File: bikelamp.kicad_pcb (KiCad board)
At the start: 2 copper layers, 56.5 x 60.1 mm, 71 parts, among them J1 Conn_ARM_SWD_TagConnect_TC203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, Q1 Q_PMOS_GSD, Q2 BSS138, Q3 RBFET, Q4 HIGH, Q5 LOW, Q6 ACFET, Q7 BSS138, Q8 YJQ3400A-YAN, Q9 YJQ3400A-YAN, SW1 SW_MEC_5E, U1 MCP79402T-xSN, U2 BQ24780SRUYR, U3 MIC5205-3.3YM5, U4 MMA8452QR1, U5 YJ-14015, U6 MC-306

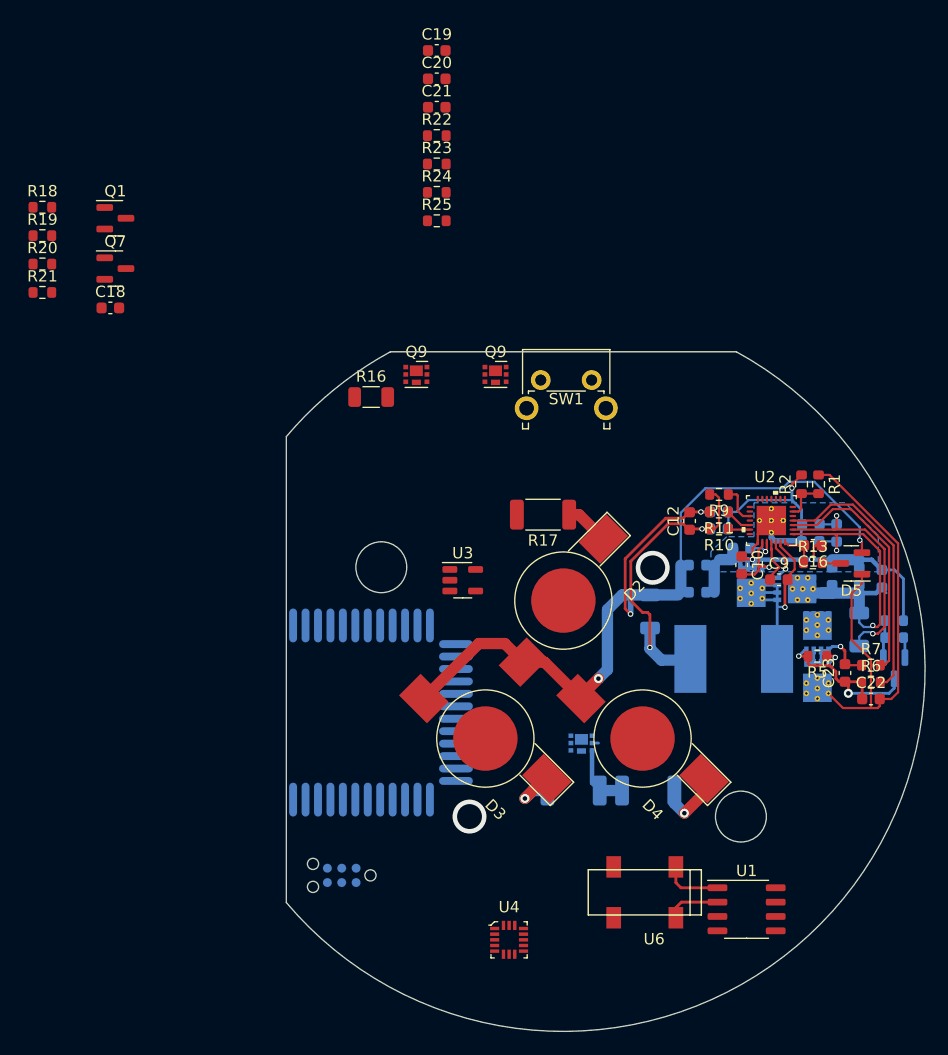
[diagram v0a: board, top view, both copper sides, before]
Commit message: Board routed
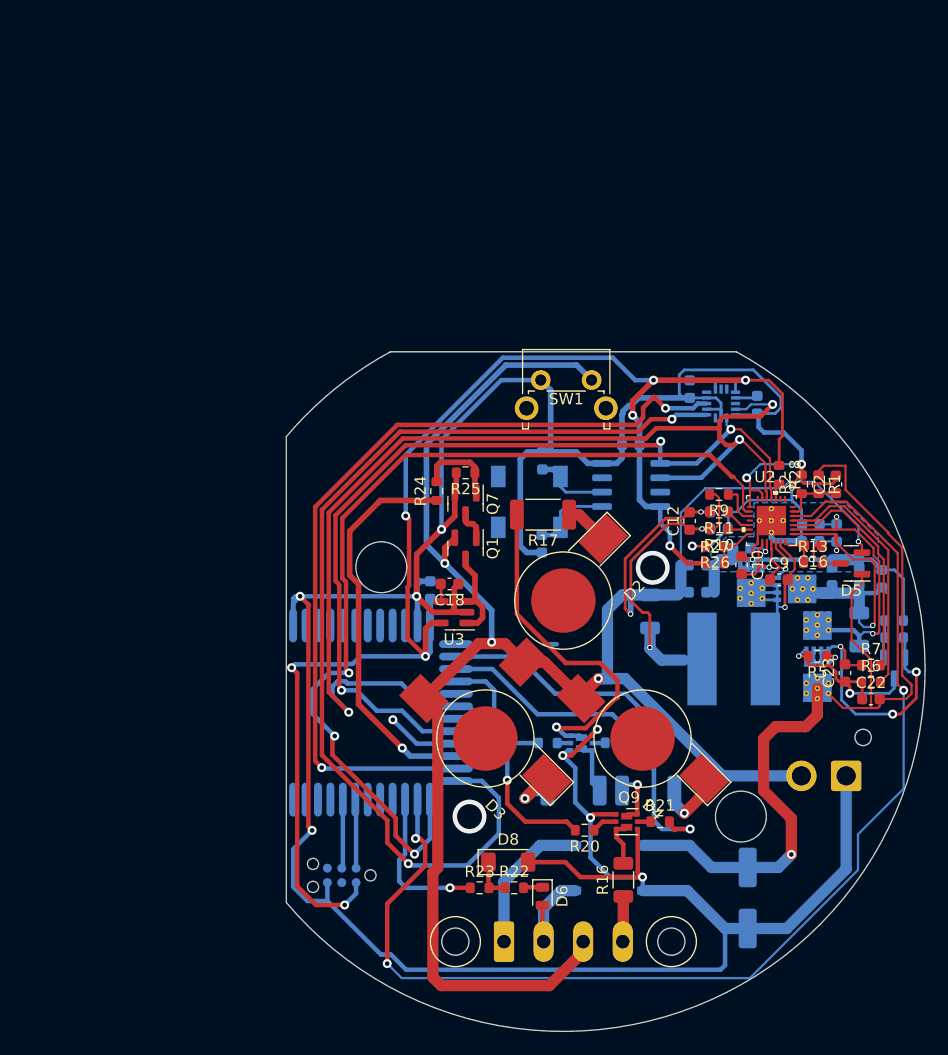
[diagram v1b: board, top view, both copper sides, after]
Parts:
- removed the Q9 at (-3.00, 2.00)
- removed the Q9 at (4.00, 2.00)
- added C1: 100uF, Capacitor_SMD:CP_Elec_6.3x5.7, B.Cu at (26.3, 48.3)
- added C2: 100nF, Capacitor_SMD:C_0603_1608Metric, F.Cu at (34.1, 11.7)
- added C24: 100nF, Capacitor_SMD:C_0603_1608Metric, B.Cu at (21.2, 3.30)
- added C25: 100nF, Capacitor_SMD:C_0603_1608Metric, B.Cu at (16.0, 8.23)
- added C26: 100nF, Capacitor_SMD:C_0603_1608Metric, B.Cu at (-1.77, 21.1)
- added D1: D_Bridge_+-AA, Diode_SMD:Diode_Bridge_Diotec_ABS, B.Cu at (14.1, 45.6)
- added D6: D_Schottky, Diode_SMD:D_MicroMELF, F.Cu at (8.15, 48.1)
- added D8: BZV55C2V7, Diode_SMD:D_MiniMELF, F.Cu at (5.12, 45.1)
- added J2: Conn_01x04_Pin, Connector_Phoenix_MC:PhoenixContact_MCV_1,5_4-GF-3.5_1x04_P3.50mm_Vertical_ThreadedFlange_MountHole, B.Cu at (4.75, 52.2)
- added J_BATTERY1: Conn_01x02, Connector_JST:JST_VH_B2P-VH-FB-B_1x02_P3.96mm_Vertical, B.Cu at (35.0, 37.5)
- added Q9: YJQ3400A-YAN, footprints:DFN2020-6L, F.Cu at (15.6, 41.5)
- added R26: TBD, Resistor_SMD:R_0603_1608Metric, F.Cu at (23.4, 17.2)
- added R27: TBD, Resistor_SMD:R_0603_1608Metric, F.Cu at (23.4, 18.7)
- added R28: 10K, Resistor_SMD:R_0603_1608Metric, F.Cu at (29.1, 10.9)
- C19, C20, C21, R18, R19, U1, U6: moved to B.Cu
- L1: footprint libs:IND_ETQP5M150YFK -> Inductor_SMD:L_Bourns-SRN8040_8x8.15mm
- Q8: footprint Package_DFN_QFN:Diodes_UDFN2020-6_Type-F -> footprints:DFN2020-6L
- U4: footprint digikey-footprints:VQFN-16_3x3mm -> footprints:VQFN-16_3x3mm; moved to B.Cu
- moved R21 71.9 mm to (18.6, 41.5)
- moved R20 69.3 mm to (11.9, 42.3), turned to 180 degrees
- moved R18 69.3 mm to (14.5, 34.6)
- moved R22 66.9 mm to (5.65, 47.4)
- moved R23 64.1 mm to (2.60, 47.4)
- moved R19 63.3 mm to (8.62, 34.6), turned to 180 degrees
- moved U4 51.0 mm to (23.9, 4.58), turned to 180 degrees
- moved R16 48.2 mm to (15.3, 46.7), turned to 90 degrees
- moved Q1 42.6 mm to (1.35, 17.4), turned to -90 degrees
- moved C19 42.2 mm to (27.1, 4.67), turned to 90 degrees
- moved C21 39.7 mm to (8.09, 17.0), turned to 90 degrees
- moved U1 38.9 mm to (16.0, 11.8)
- moved C18 38.7 mm to (-0.07, 20.5), turned to 180 degrees
- moved Q7 37.3 mm to (1.35, 13.4), turned to -90 degrees
- moved U6 36.0 mm to (6.99, 13.3)
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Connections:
- net /BQ24780/ACN renamed /BQ24780/VIN_I_MEASURED
- net /BQ24780/ACP renamed /BQ24780/VIN_REVPROT
- R16 pad 1: Net-(J_REAR_LAMP1-Pin_1) -> REAR_LAMP_K
- U2 pad 10: unconnected-(U2-PROCHOT_N-Pad10) -> Net-(U2-PROCHOT_N)
- U2 pad 13: unconnected-(U2-CMPIN-Pad13) -> GND
- U2 pad 15: unconnected-(U2-BATPRES_N-Pad15) -> GND
- U2 pad 16: unconnected-(U2-TB_STAT_N-Pad16) -> TB_STAT
- U2 pad 21: unconnected-(U2-ILIM-Pad21) -> /BQ24780/ILIM
- U2 pad 5: unconnected-(U2-ACOK-Pad5) -> ACOK
- U5 pad 15: LED_PWM_1 -> LED_PWM_0
- U5 pad 16: LED_PWM_0 -> LED_PWM_1
- U5 pad 17: WHEEL_SIGNAL -> unconnected-(U5-P03-Pad17)
- U5 pad 25: unconnected-(U5-P11-Pad25) -> TB_STAT
- U5 pad 26: unconnected-(U5-P12-Pad26) -> ACOK
- U5 pad 27: unconnected-(U5-P13-Pad27) -> WHEEL_SIGNAL
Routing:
- net GND: track 15.3 -> 307.7 mm, vias 1 -> 12
- net +3V3: track 0.00 -> 141.1 mm, vias 0 -> 8
- net ACOK: track 0.00 -> 104.3 mm, vias 0 -> 3
- net VBAT: track 64.1 -> 168.1 mm, vias 2 -> 4
- net SCL: track 0.00 -> 98.8 mm, vias 0 -> 3
- net MMA8452_INT2: track 0.00 -> 88.8 mm, vias 0 -> 2
- net TB_STAT: track 0.00 -> 83.3 mm, vias 0 -> 3
- net SDA: track 0.00 -> 77.6 mm, vias 0 -> 3
- net MMA8452_INT1: track 0.00 -> 74.9 mm, vias 0 -> 2
- net VDD: track 43.3 -> 80.9 mm, vias 0 -> 1
- net KEEP_POWER: track 0.00 -> 35.0 mm, vias 0 -> 1
- net LED_PWM_2: track 0.00 -> 34.5 mm, vias 0 -> 1
- net Net-(Q8A-D): track 0.00 -> 30.8 mm, vias 0 -> 1
- net LED_PWM_0: track 0.00 -> 18.4 mm
- net LED_PWM_3: track 0.00 -> 18.1 mm, vias 0 -> 1
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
